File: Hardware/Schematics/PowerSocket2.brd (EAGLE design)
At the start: 99 x 48.5 mm, 80 parts, among them IC1 REG1117, IC3 74AC373DW, J1 1X2-3.5MM, J2 1X2-3.5MM, J3 1X2-3.5MM, J4 1X2-3.5MM, J5 1X2-3.5MM, J6 1X2-3.5MM, J7 1X2-3.5MM, J8 1X2-3.5MM, J9 1X2-3.5MM, U1 ESP-32S

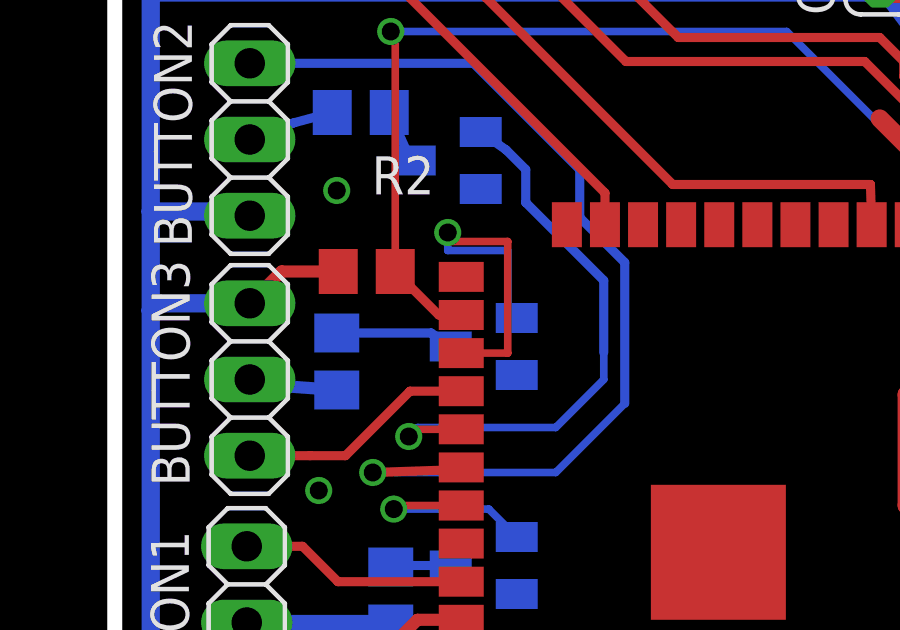
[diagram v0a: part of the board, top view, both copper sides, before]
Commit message: Return OK in settings.
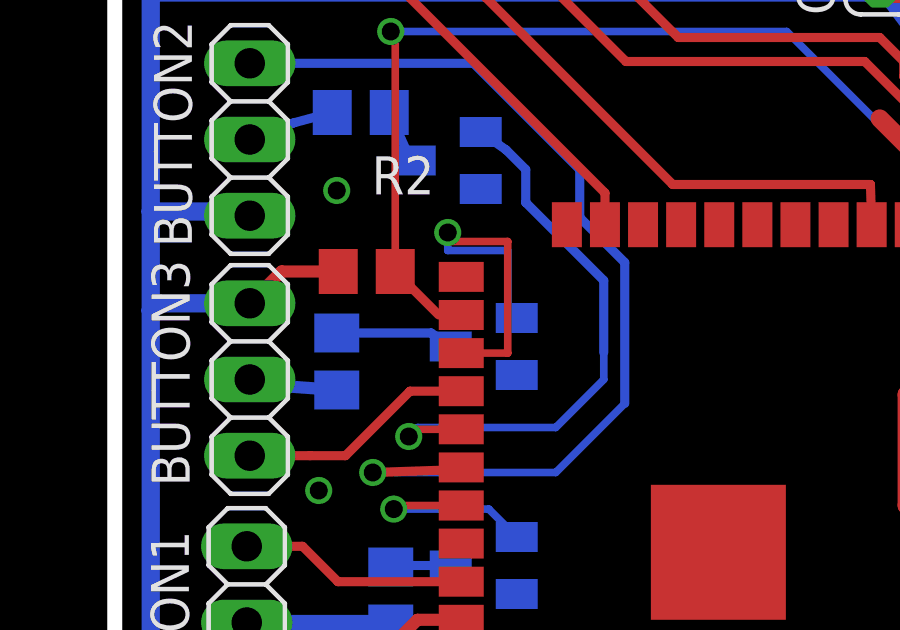
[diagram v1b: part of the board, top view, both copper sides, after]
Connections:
- net FLASH: now also U1.25; no longer U1.26
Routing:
- net FLASH: track 54.9 -> 54.1 mm
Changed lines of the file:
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@@
 <contactref element="R2" pad="2"/>
 <contactref element="FLASH" pad="3"/>
-<contactref element="U1" pad="26"/>
-<wire x1="11.3" y1="30.15" x2="12.05" y2="30.15" width="0.3048" layer="1"/>
 <wire x1="9.85" y1="31.6" x2="11.3" y2="30.15" width="0.3048" layer="1"/>
 <wire x1="49.0512" y1="38.2394" x2="42.5488" y2="38.2394" width="0.3048" layer="16"/>
@@
 <wire x1="29.2" y1="33.3" x2="22.9" y2="39.6" width="0.254" layer="16"/>
 <wire x1="22.9" y1="39.6" x2="9.7" y2="39.6" width="0.254" layer="16"/>
+<contactref element="U1" pad="25"/>
+<wire x1="11.3" y1="30.15" x2="12.05" y2="31.42" width="0" layer="19" extent="1-1"/>
 </signal>
 <signal name="GATE3">
